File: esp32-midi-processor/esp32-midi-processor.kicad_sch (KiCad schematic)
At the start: 23 parts, among them J1 Midi IN 1, J2 Midi IN 2, J3 Midi OUT 1, J4 Midi OUT 2, J5 Conn_01x15_Socket, J6 Conn_01x15_Socket, J7 Input Voltage, U1 6N138, U2 6N138

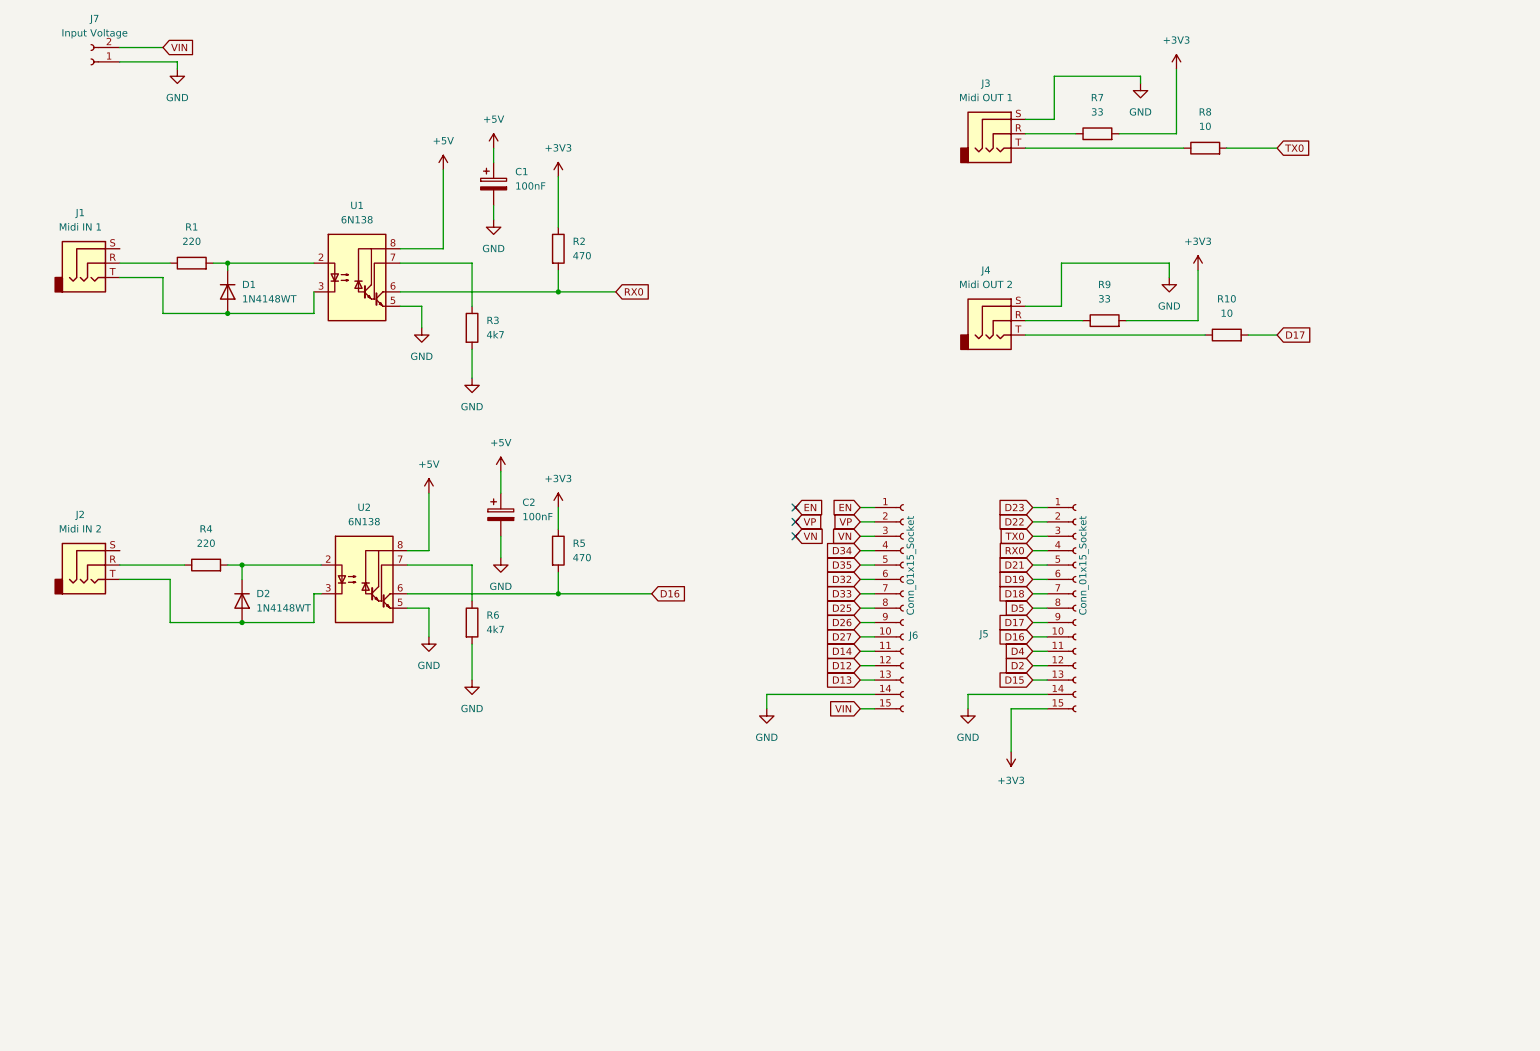
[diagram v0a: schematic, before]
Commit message: add more stuff to schematic
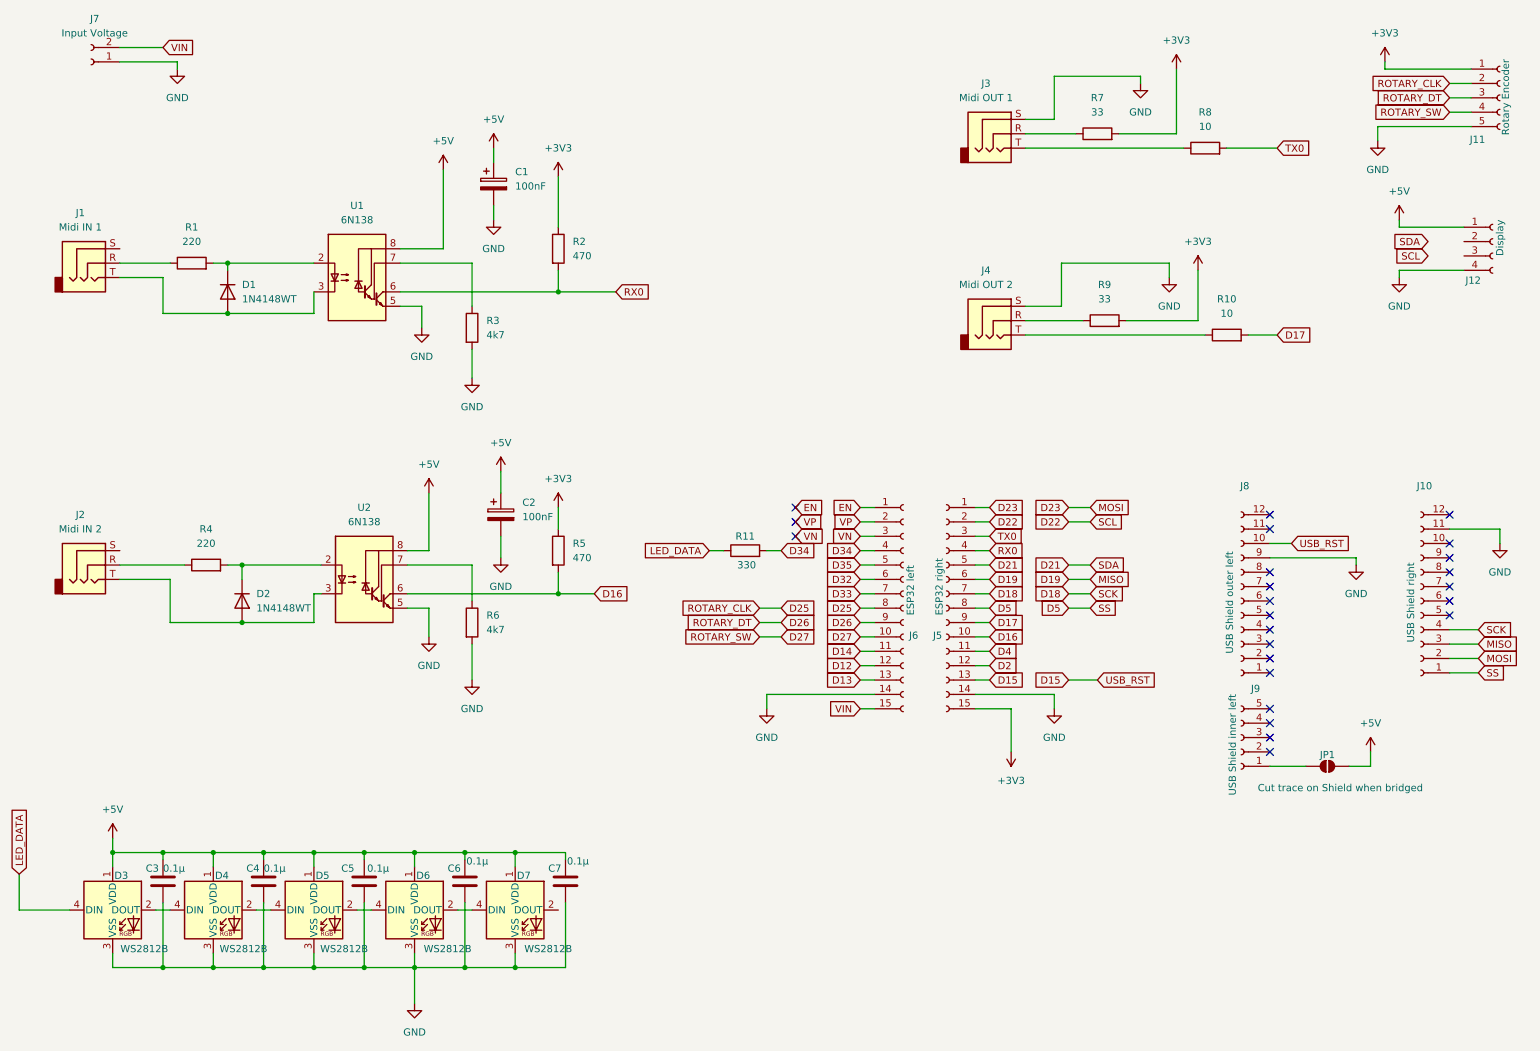
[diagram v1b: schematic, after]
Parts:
- added C3, C4, C5, C6, C7: 0.1µ, Capacitor_SMD:C_0603_1608Metric, symbol Device:C
- added D3, D4, D5, D6, D7: WS2812B, LED_SMD:LED_WS2812B_PLCC4_5.0x5.0mm_P3.2mm, symbol LED:WS2812B
- added J10: USB Shield right, symbol Connector:Conn_01x12_Socket
- added J11: Rotary Encoder, symbol Connector:Conn_01x05_Socket
- added J12: Display, symbol Connector:Conn_01x04_Socket
- added J8: USB Shield outer left, symbol Connector:Conn_01x12_Socket
- added J9: USB Shield inner left, symbol Connector:Conn_01x05_Socket
- added JP1: Cut trace on Shield when bridged, symbol Jumper:SolderJumper_2_Open
- added R11: 330, symbol Device:R
- J5: value Conn_01x15_Socket -> ESP32 right
- J6: value Conn_01x15_Socket -> ESP32 left
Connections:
- net +3V3: now also J11.1 (Pin_1)
- net +5V: now also C3.1, C4.1, C5.1, C6.1, C7.1, D3.1 (VDD), D4.1 (VDD), D5.1 (VDD), D6.1 (VDD), D7.1 (VDD), J12.1 (Pin_1), JP1.2 (B)
- net D15: now also J8.10 (Pin_10)
- net D18: now also J10.4 (Pin_4)
- net D19: now also J10.3 (Pin_3)
- net D23: now also J10.2 (Pin_2)
- net D25: now also J11.2 (Pin_2)
- net D26: now also J11.3 (Pin_3)
- net D27: now also J11.4 (Pin_4)
- net D34: now also R11.2
- net D5: now also J10.1 (Pin_1)
- net GND: now also C3.2, C4.2, C5.2, C6.2, C7.2, D3.3 (VSS), D4.3 (VSS), D5.3 (VSS), D6.3 (VSS), D7.3 (VSS), J10.11 (Pin_11), J11.5 (Pin_5), J12.4 (Pin_4), J8.9 (Pin_9)
- new net: D5.2 (DOUT), D6.4 (DIN)
- new net: D4.2 (DOUT), D5.4 (DIN)
- new net: J9.1 (Pin_1), JP1.1 (A)
- new net: D3.2 (DOUT), D4.4 (DIN)
- new net: D6.2 (DOUT), D7.4 (DIN)
- new net LED_DATA: D3.4 (DIN), R11.1
- no-connect marks 3 -> 24
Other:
- moved on the sheet: J5
